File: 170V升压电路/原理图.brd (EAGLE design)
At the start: 100 x 80 mm, 20 parts, among them IC1 MC34063AP

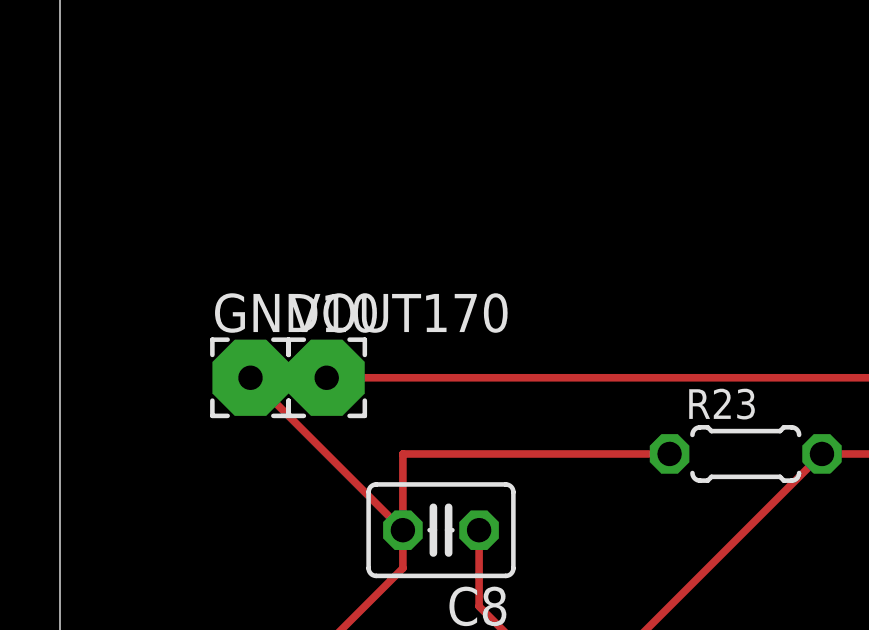
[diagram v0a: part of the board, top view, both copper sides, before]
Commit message: 优化
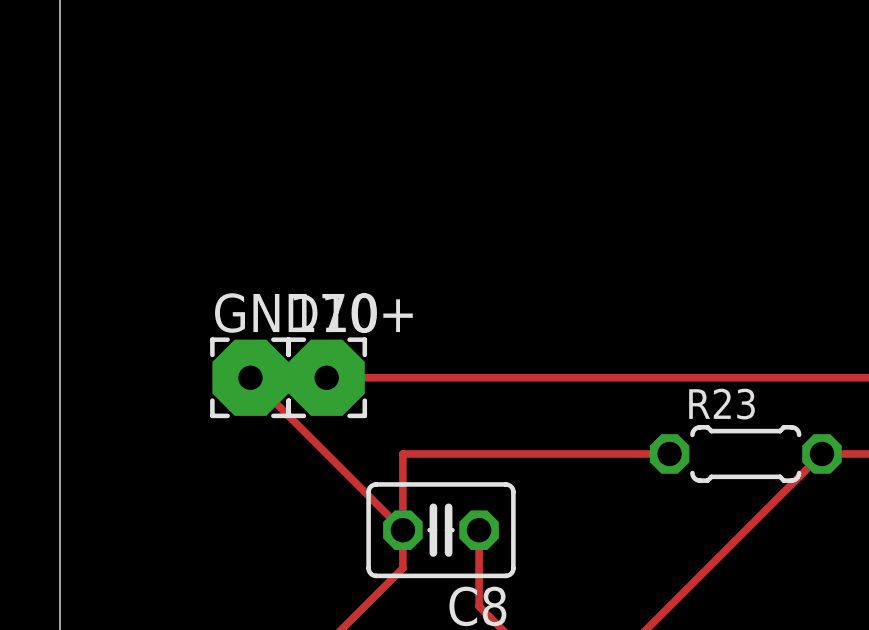
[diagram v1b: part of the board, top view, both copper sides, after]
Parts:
- renumbered VOUT170 to 170+
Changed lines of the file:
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@@
 <layer number="17" name="Pads" color="2" fill="1" visible="yes" active="yes"/>
 <layer number="18" name="Vias" color="2" fill="1" visible="yes" active="yes"/>
-<layer number="19" name="Unrouted" color="6" fill="1" visible="no" active="yes"/>
-<layer number="20" name="Dimension" color="15" fill="1" visible="no" active="yes"/>
-<layer number="21" name="tPlace" color="7" fill="1" visible="no" active="yes"/>
-<layer number="22" name="bPlace" color="7" fill="1" visible="no" active="yes"/>
-<layer number="23" name="tOrigins" color="15" fill="1" visible="no" active="yes"/>
-<layer number="24" name="bOrigins" color="15" fill="1" visible="no" active="yes"/>
-<layer number="25" name="tNames" color="7" fill="1" visible="no" active="yes"/>
-<layer number="26" name="bNames" color="7" fill="1" visible="no" active="yes"/>
-<layer number="27" name="tValues" color="7" fill="1" visible="no" active="yes"/>
-<layer number="28" name="bValues" color="7" fill="1" visible="no" active="yes"/>
-<layer number="29" name="tStop" color="7" fill="3" visible="no" active="yes"/>
-<layer number="30" name="bStop" color="7" fill="6" visible="no" active="yes"/>
-<layer number="31" name="tCream" color="7" fill="4" visible="no" active="yes"/>
-<layer number="32" name="bCream" color="7" fill="5" visible="no" active="yes"/>
-<layer number="33" name="tFinish" color="6" fill="3" visible="no" active="yes"/>
-<layer number="34" name="bFinish" color="6" fill="6" visible="no" active="yes"/>
-<layer number="35" name="tGlue" color="7" fill="4" visible="no" active="yes"/>
-<layer number="36" name="bGlue" color="7" fill="5" visible="no" active="yes"/>
-<layer number="37" name="tTest" color="7" fill="1" visible="no" active="yes"/>
-<layer number="38" name="bTest" color="7" fill="1" visible="no" active="yes"/>
-<layer number="39" name="tKeepout" color="4" fill="11" visible="no" active="yes"/>
-<layer number="40" name="bKeepout" color="1" fill="11" visible="no" active="yes"/>
-<layer number="41" name="tRestrict" color="4" fill="10" visible="no" active="yes"/>
-<layer number="42" name="bRestrict" color="1" fill="10" visible="no" active="yes"/>
-<layer number="43" name="vRestrict" color="2" fill="10" visible="no" active="yes"/>
-<layer number="44" name="Drills" color="7" fill="1" visible="no" active="yes"/>
-<layer number="45" name="Holes" color="7" fill="1" visible="no" active="yes"/>
-<layer number="46" name="Milling" color="3" fill="1" visible="no" active="yes"/>
-<layer number="47" name="Measures" color="7" fill="1" visible="no" active="yes"/>
-<layer number="48" name="Document" color="7" fill="1" visible="no" active="yes"/>
-<layer number="49" name="Reference" color="7" fill="1" visible="no" active="yes"/>
+<layer number="19" name="Unrouted" color="6" fill="1" visible="yes" active="yes"/>
+<layer number="20" name="Dimension" color="15" fill="1" visible="yes" active="yes"/>
+<layer number="21" name="tPlace" color="7" fill="1" visible="yes" active="yes"/>
+<layer number="22" name="bPlace" color="7" fill="1" visible="yes" active="yes"/>
+<layer number="23" name="tOrigins" color="15" fill="1" visible="yes" active="yes"/>
+<layer number="24" name="bOrigins" color="15" fill="1" visible="yes" active="yes"/>
+<layer number="25" name="tNames" color="7" fill="1" visible="yes" active="yes"/>
+<layer number="26" name="bNames" color="7" fill="1" visible="yes" active="yes"/>
+<layer number="27" name="tValues" color="7" fill="1" visible="yes" active="yes"/>
+<layer number="28" name="bValues" color="7" fill="1" visible="yes" active="yes"/>
+<layer number="29" name="tStop" color="7" fill="3" visible="yes" active="yes"/>
+<layer number="30" name="bStop" color="7" fill="6" visible="yes" active="yes"/>
+<layer number="31" name="tCream" color="7" fill="4" visible="yes" active="yes"/>
+<layer number="32" name="bCream" color="7" fill="5" visible="yes" active="yes"/>
+<layer number="33" name="tFinish" color="6" fill="3" visible="yes" active="yes"/>
+<layer number="34" name="bFinish" color="6" fill="6" visible="yes" active="yes"/>
+<layer number="35" name="tGlue" color="7" fill="4" visible="yes" active="yes"/>
+<layer number="36" name="bGlue" color="7" fill="5" visible="yes" active="yes"/>
+<layer number="37" name="tTest" color="7" fill="1" visible="yes" active="yes"/>
+<layer number="38" name="bTest" color="7" fill="1" visible="yes" active="yes"/>
+<layer number="39" name="tKeepout" color="4" fill="11" visible="yes" active="yes"/>
+<layer number="40" name="bKeepout" color="1" fill="11" visible="yes" active="yes"/>
+<layer number="41" name="tRestrict" color="4" fill="10" visible="yes" active="yes"/>
+<layer number="42" name="bRestrict" color="1" fill="10" visible="yes" active="yes"/>
+<layer number="43" name="vRestrict" color="2" fill="10" visible="yes" active="yes"/>
+<layer number="44" name="Drills" color="7" fill="1" visible="yes" active="yes"/>
+<layer number="45" name="Holes" color="7" fill="1" visible="yes" active="yes"/>
+<layer number="46" name="Milling" color="3" fill="1" visible="yes" active="yes"/>
+<layer number="47" name="Measures" color="7" fill="1" visible="yes" active="yes"/>
+<layer number="48" name="Document" color="7" fill="1" visible="yes" active="yes"/>
+<layer number="49" name="Reference" color="7" fill="1" visible="yes" active="yes"/>
 <layer number="50" name="dxf" color="7" fill="1" visible="no" active="no"/>
-<layer number="51" name="tDocu" color="7" fill="1" visible="no" active="yes"/>
-<layer number="52" name="bDocu" color="7" fill="1" visible="no" active="yes"/>
+<layer number="51" name="tDocu" color="7" fill="1" visible="yes" active="yes"/>
+<layer number="52" name="bDocu" color="7" fill="1" visible="yes" active="yes"/>
 <layer number="91" name="Nets" color="2" fill="1" visible="no" active="no"/>
 <layer number="92" name="Busses" color="1" fill="1" visible="no" active="no"/>
@@
 <layer number="97" name="Info" color="7" fill="1" visible="no" active="no"/>
 <layer number="98" name="Guide" color="6" fill="1" visible="no" active="no"/>
-<layer number="200" name="200bmp" color="7" fill="1" visible="no" active="yes"/>
-<layer number="231" name="Eagle3D_PG1" color="7" fill="1" visible="no" active="yes"/>
-<layer number="232" name="Eagle3D_PG2" color="7" fill="1" visible="no" active="yes"/>
-<layer number="233" name="Eagle3D_PG3" color="7" fill="1" visible="no" active="yes"/>
-<layer number="250" name="Descript" color="7" fill="1" visible="no" active="yes"/>
-<layer number="251" name="SMDround" color="7" fill="1" visible="no" active="yes"/>
+<layer number="200" name="200bmp" color="7" fill="1" visible="yes" active="yes"/>
+<layer number="231" name="Eagle3D_PG1" color="7" fill="1" visible="yes" active="yes"/>
+<layer number="232" name="Eagle3D_PG2" color="7" fill="1" visible="yes" active="yes"/>
+<layer number="233" name="Eagle3D_PG3" color="7" fill="1" visible="yes" active="yes"/>
+<layer number="250" name="Descript" color="7" fill="1" visible="yes" active="yes"/>
+<layer number="251" name="SMDround" color="7" fill="1" visible="yes" active="yes"/>
 </layers>
 <board>
@@
 <attribute name="VALUE" x="7.62" y="5.68" size="0.0254" layer="27"/>
 </element>
-<element name="VOUT170" library="wirepad" package="2,54/0,8" value="" x="8.89" y="38.1" smashed="yes">
+<element name="170+" library="wirepad" package="2,54/0,8" value="" x="8.89" y="38.1" smashed="yes">
 <attribute name="NAME" x="7.62" y="39.624" size="1.27" layer="25" ratio="10"/>
 <attribute name="VALUE" x="8.89" y="38.7" size="0.0254" layer="27"/>
@@
 <contactref element="VD3" pad="C"/>
 <contactref element="C5" pad="1"/>
-<contactref element="VOUT170" pad="1"/>
+<contactref element="170+" pad="1"/>
 <wire x1="40.64" y1="30.48" x2="35.56" y2="35.56" width="0.254" layer="1"/>
 <wire x1="48.26" y1="30.48" x2="40.64" y2="30.48" width="0.254" layer="1"/>
